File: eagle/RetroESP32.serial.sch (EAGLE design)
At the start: 70 parts, among them J1 AUDIO_JACK_3.5MM_KIT, J2 SPKR, J3 Batt Conn, J5 503182-1852_503182-1852, J6 USB4110-GF-A, Q3 DMG3415U-7, Q4 mmbt2222, Q5 mmbt2222, U1 ESP32-WROVER_ESP32-WROVER, U3 XC6210B332MR-G, U4 MCP73832T-2ACI/OT, U6 LM4875

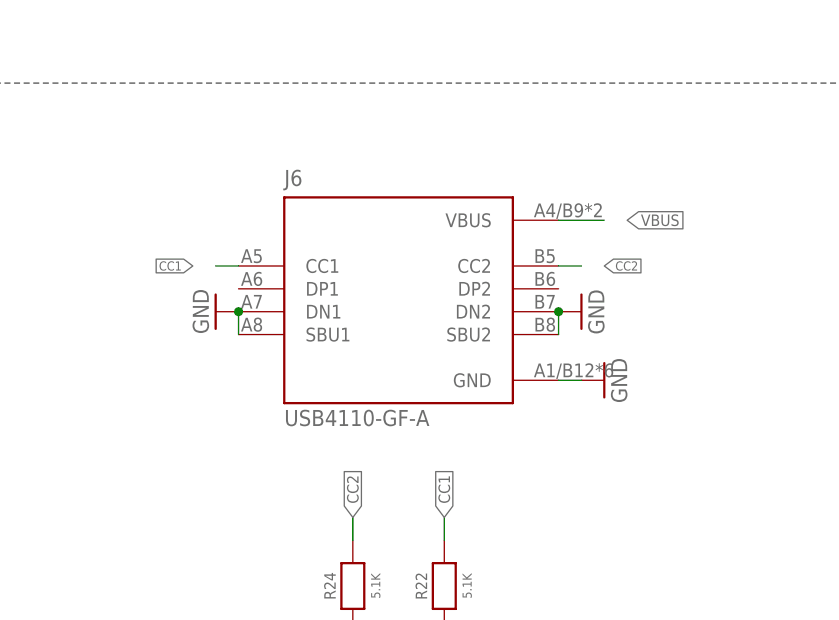
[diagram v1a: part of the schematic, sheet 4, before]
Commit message: feat: new button library
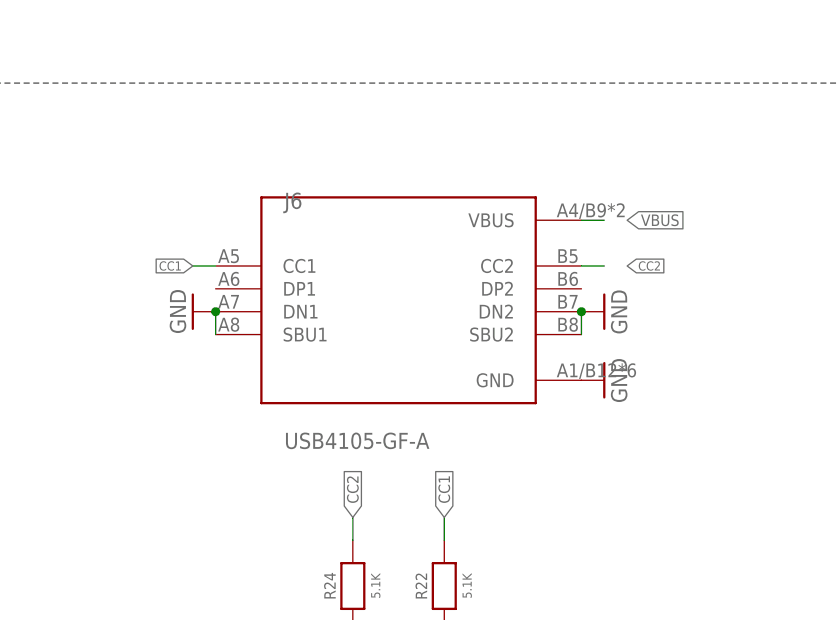
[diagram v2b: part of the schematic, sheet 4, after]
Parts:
- DOWN, LEFT, RIGHT, UP: value CONDUCTIVE_BUTTONCONDUCTIVE_BUTTON_DIRECTIONAL_THICK -> CONDUCTIVE_BUTTON; device RetroESP32:CONDUCTIVE_BUTTONCONDUCTIVE_BUTTON_DIRECTIONAL_THICK -> RetroESP32:CONDUCTIVE_BUTTON
- J6: value USB4110-GF-A -> USB4105-GF-A; device USB4110-GF-A:USB4110-GF-A -> RetroESP32:USB4105-GF-A

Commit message: feat: new A/B buttons, osh gerber
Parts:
- A: value CONDUCTIVE_BUTTONCONDUCTIVE_BUTTON_THICK -> CONDUCTIVE_BUTTONCONDUCTIVE_BUTTON_MGB; device RetroESP32:CONDUCTIVE_BUTTONCONDUCTIVE_BUTTON_THICK -> RetroESP32:CONDUCTIVE_BUTTONCONDUCTIVE_BUTTON_MGB
- B: value CONDUCTIVE_BUTTONCONDUCTIVE_BUTTON_THICK -> CONDUCTIVE_BUTTONCONDUCTIVE_BUTTON_MGB; device RetroESP32:CONDUCTIVE_BUTTONCONDUCTIVE_BUTTON_THICK -> RetroESP32:CONDUCTIVE_BUTTONCONDUCTIVE_BUTTON_MGB; SPICEPREFIX (none) -> B
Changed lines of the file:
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@@
 <part name="U$9" library="RetroESP32" library_urn="urn:adsk.eagle:library:12566846" deviceset="GND" device=""/>
 <part name="U$10" library="RetroESP32" library_urn="urn:adsk.eagle:library:12566846" deviceset="GND" device=""/>
-<part name="B" library="RetroESP32" library_urn="urn:adsk.eagle:library:12566846" deviceset="CONDUCTIVE_BUTTON" device="CONDUCTIVE_BUTTON_THICK" package3d_urn="urn:adsk.eagle:package:12566912/6" value="CONDUCTIVE_BUTTONCONDUCTIVE_BUTTON_THICK">
+<part name="B" library="RetroESP32" library_urn="urn:adsk.eagle:library:12566846" deviceset="CONDUCTIVE_BUTTON" device="CONDUCTIVE_BUTTON_MGB" value="CONDUCTIVE_BUTTONCONDUCTIVE_BUTTON_MGB">
 <attribute name="IGNORE_BOM" value="TRUE"/>
+<attribute name="SPICEPREFIX" value="B"/>
 </part>
 <part name="START" library="RetroESP32" library_urn="urn:adsk.eagle:library:12566846" deviceset="CONDUCTIVE_BUTTON_STARTSELECT" device="CONDUCTIVE_BUTTON_THICK_STARTSELECT" package3d_urn="urn:adsk.eagle:package:12566911/5" value="CONDUCTIVE_BUTTON_STARTSELECTCONDUCTIVE_BUTTON_THICK_STARTSELECT">
@@
 <attribute name="IGNORE_BOM" value="TRUE"/>
 </part>
-<part name="A" library="RetroESP32" library_urn="urn:adsk.eagle:library:12566846" deviceset="CONDUCTIVE_BUTTON" device="CONDUCTIVE_BUTTON_THICK" package3d_urn="urn:adsk.eagle:package:12566912/6" value="CONDUCTIVE_BUTTONCONDUCTIVE_BUTTON_THICK">
+<part name="A" library="RetroESP32" library_urn="urn:adsk.eagle:library:12566846" deviceset="CONDUCTIVE_BUTTON" device="CONDUCTIVE_BUTTON_MGB" value="CONDUCTIVE_BUTTONCONDUCTIVE_BUTTON_MGB">
 <attribute name="IGNORE_BOM" value="TRUE"/>
 </part>
-<part name="UP" library="RetroESP32" library_urn="urn:adsk.eagle:library:12566846" deviceset="CONDUCTIVE_BUTTON" device="" value="CONDUCTIVE_BUTTON">
+<part name="UP" library="RetroESP32" library_urn="urn:adsk.eagle:library:12566846" deviceset="CONDUCTIVE_BUTTON" device="" package3d_urn="urn:adsk.eagle:package:40166519/1" value="CONDUCTIVE_BUTTON">
 <attribute name="IGNORE_BOM" value="TRUE"/>
 </part>
-<part name="DOWN" library="RetroESP32" library_urn="urn:adsk.eagle:library:12566846" deviceset="CONDUCTIVE_BUTTON" device="" value="CONDUCTIVE_BUTTON">
+<part name="DOWN" library="RetroESP32" library_urn="urn:adsk.eagle:library:12566846" deviceset="CONDUCTIVE_BUTTON" device="" package3d_urn="urn:adsk.eagle:package:40166519/1" value="CONDUCTIVE_BUTTON">
 <attribute name="IGNORE_BOM" value="TRUE"/>
 </part>
-<part name="LEFT" library="RetroESP32" library_urn="urn:adsk.eagle:library:12566846" deviceset="CONDUCTIVE_BUTTON" device="" value="CONDUCTIVE_BUTTON">
+<part name="LEFT" library="RetroESP32" library_urn="urn:adsk.eagle:library:12566846" deviceset="CONDUCTIVE_BUTTON" device="" package3d_urn="urn:adsk.eagle:package:40166519/1" value="CONDUCTIVE_BUTTON">
 <attribute name="IGNORE_BOM" value="TRUE"/>
 </part>
-<part name="RIGHT" library="RetroESP32" library_urn="urn:adsk.eagle:library:12566846" deviceset="CONDUCTIVE_BUTTON" device="" value="CONDUCTIVE_BUTTON">
+<part name="RIGHT" library="RetroESP32" library_urn="urn:adsk.eagle:library:12566846" deviceset="CONDUCTIVE_BUTTON" device="" package3d_urn="urn:adsk.eagle:package:40166519/1" value="CONDUCTIVE_BUTTON">
 <attribute name="IGNORE_BOM" value="TRUE"/>
 </part>
